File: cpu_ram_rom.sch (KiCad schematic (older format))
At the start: 14 parts, among them U12 74HCT3G04, U4 Z84C0010AEG, U5 IS62C5128BL-45TLI, U6 SST39SF040

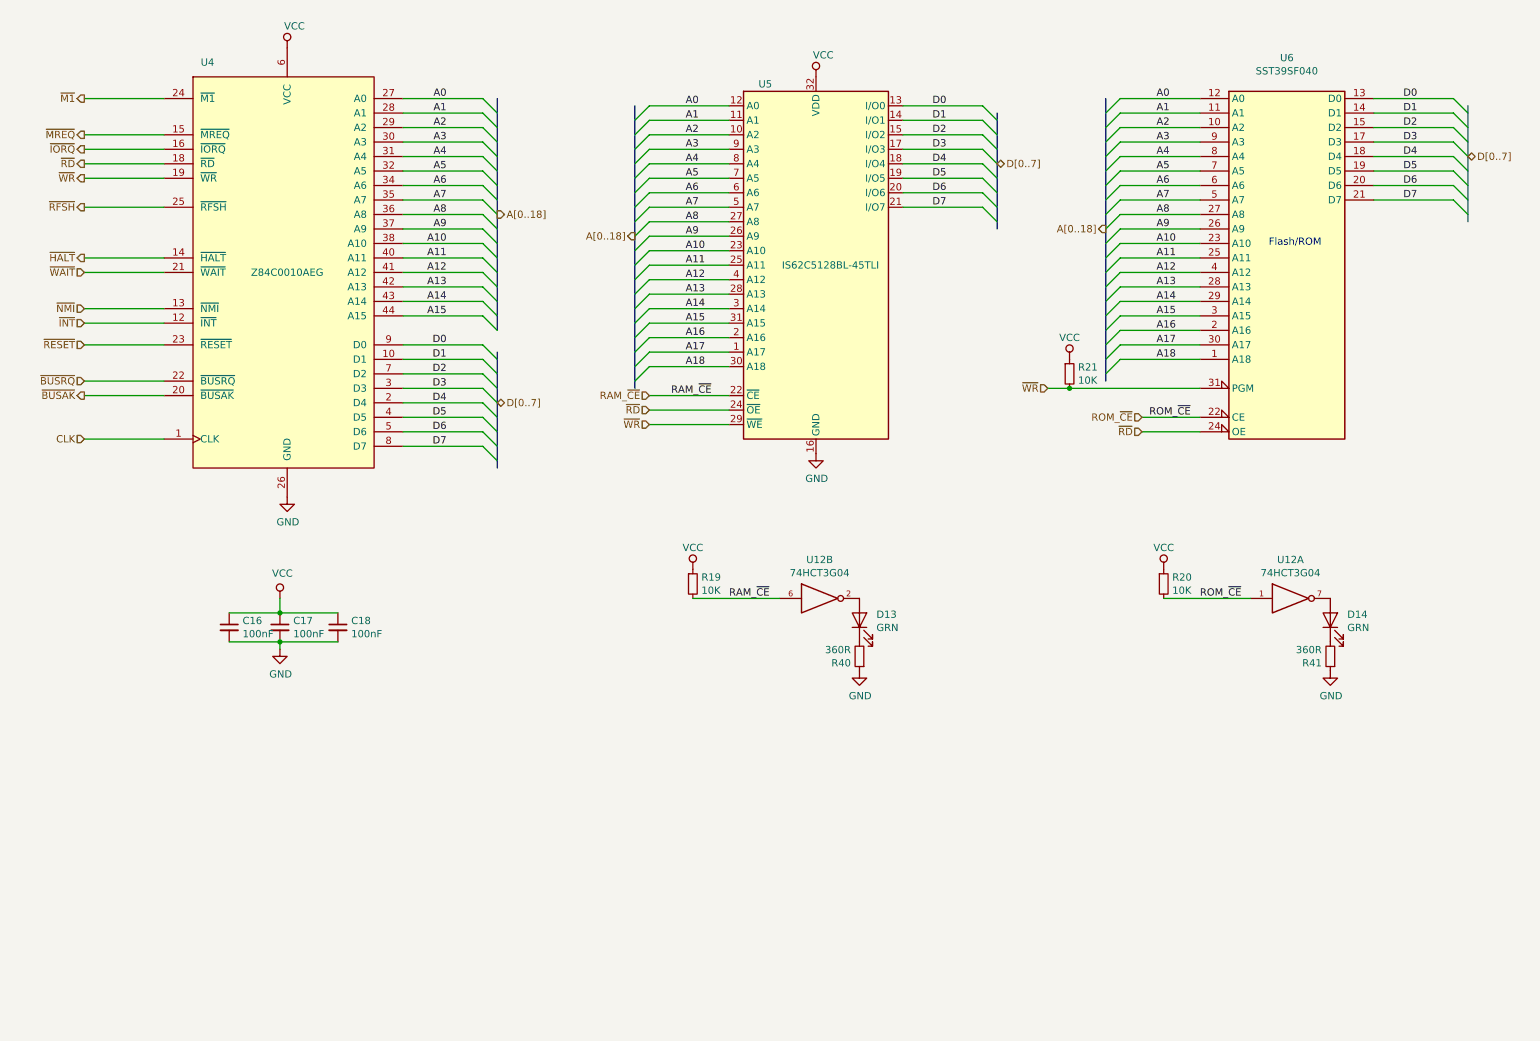
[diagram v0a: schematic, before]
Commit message: lots of fixes
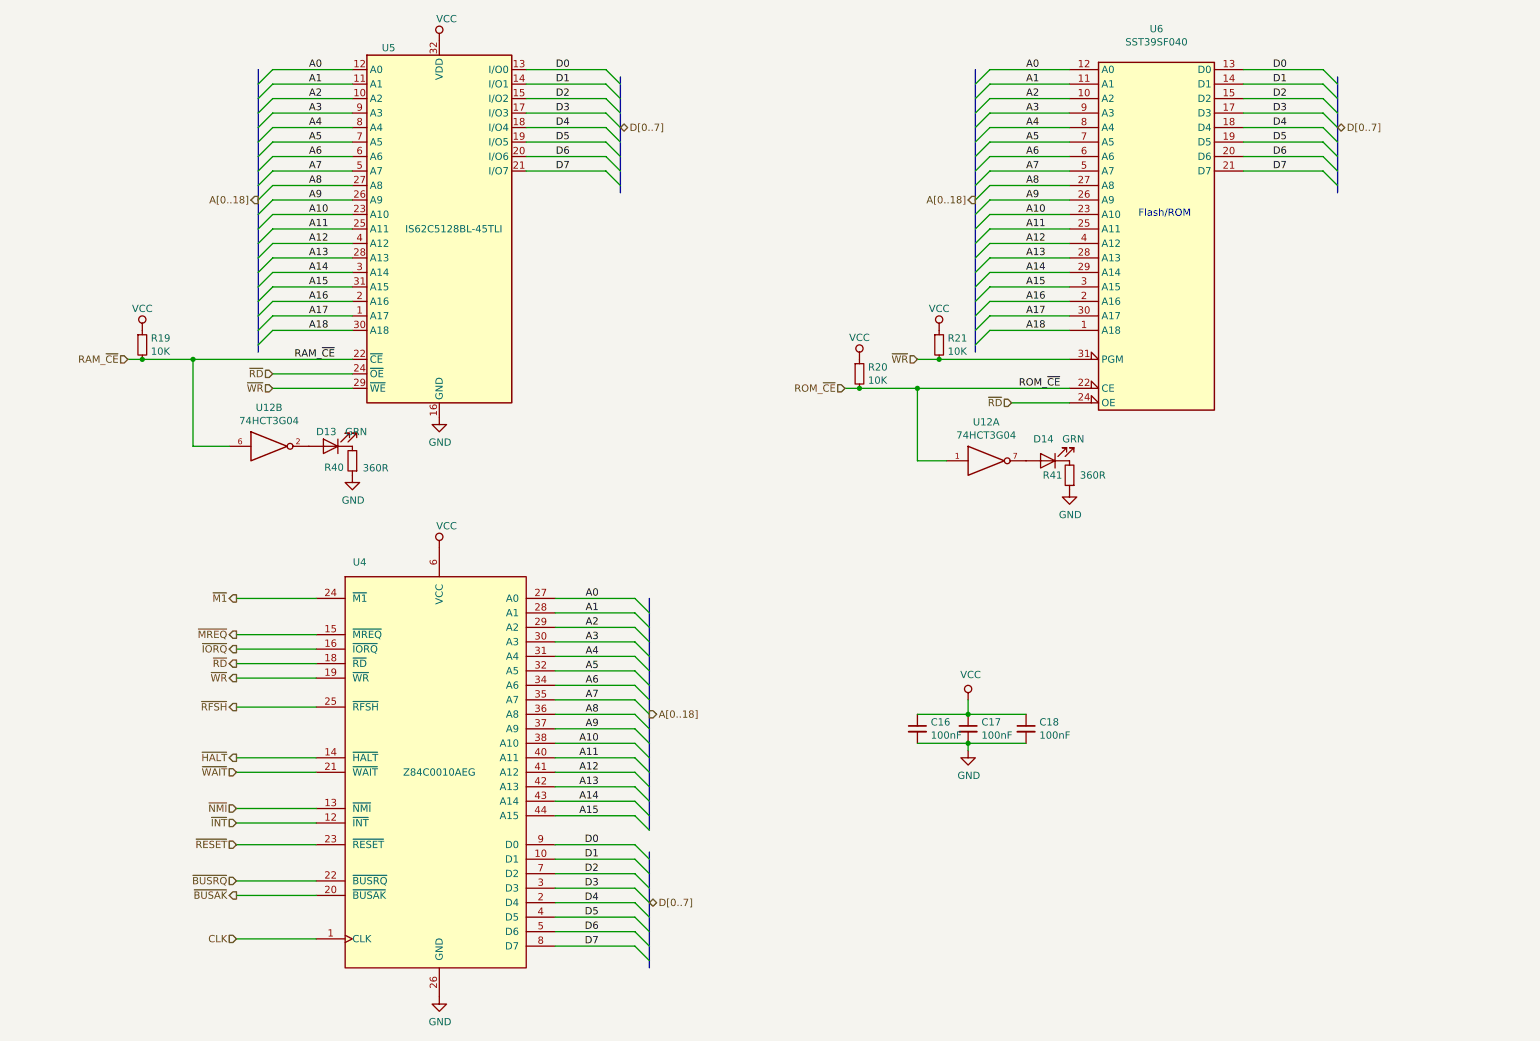
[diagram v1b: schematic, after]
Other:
- moved on the sheet: C16, C17, C18, D13, D14, R19, R20, R21, R40, R41, U12A, U12B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
